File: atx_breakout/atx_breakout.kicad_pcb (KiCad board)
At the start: 2 copper layers, 90 x 60 mm, 18 parts, among them J1 Conn_02x04_Top_Bottom, J10 Screw_Terminal_01x08, J2 Conn_02x04_Top_Bottom, J3 Conn_02x04_Top_Bottom, J4 Conn_02x04_Top_Bottom, J5 ATX-24, J6 Screw_Terminal_01x08, J7 Screw_Terminal_01x08, J8 Screw_Terminal_01x08, J9 Screw_Terminal_01x08, U1 SW_DPDT_PS-70N

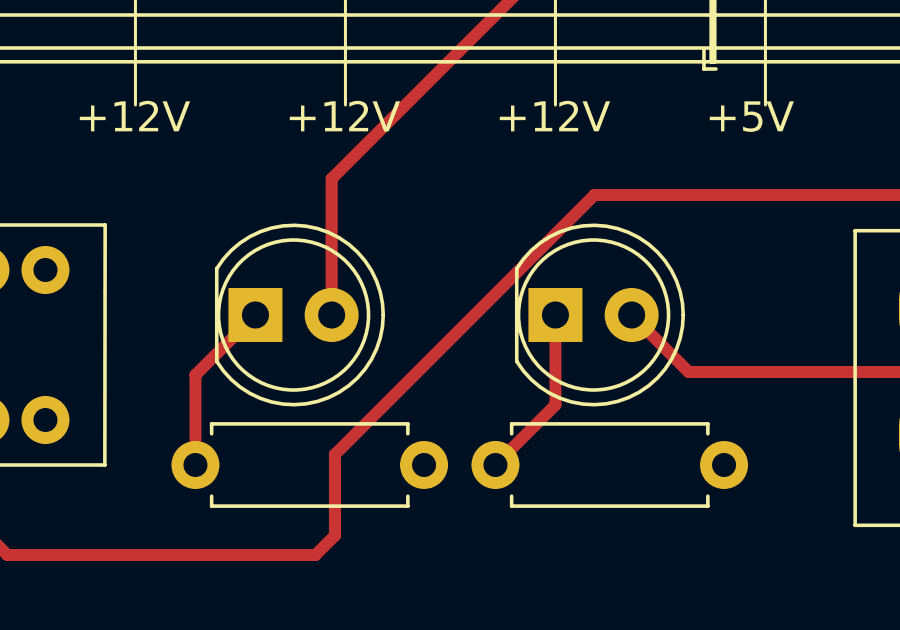
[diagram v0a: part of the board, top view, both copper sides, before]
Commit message: Update ledplane
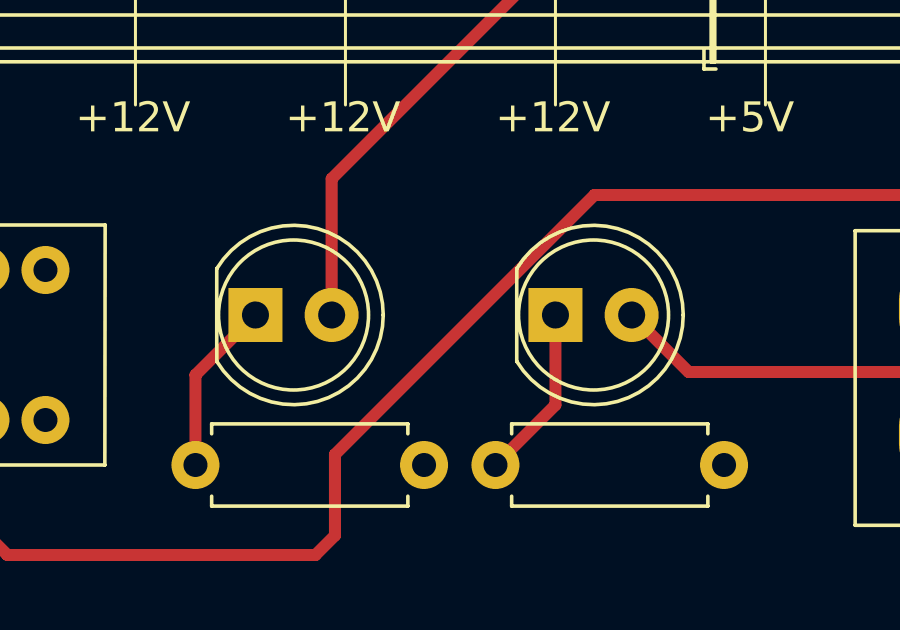
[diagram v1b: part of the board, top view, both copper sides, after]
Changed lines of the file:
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@@
 		(layer "F.Cu")
 		(at 26 17)
-		(descr "LED, diameter 5.0mm, 2 pins, http://cdn-reichelt.de/documents/datenblatt/A500/LL-504BC2E-009.pdf")
-		(tags "LED diameter 5.0mm 2 pins")
+		(descr "LED, diameter 5.0mm, 2 pins, http://cdn-reichelt.de/documents/datenblatt/A500/LL-504BC2E-009.pdf, generated by kicad-footprint-generator")
+		(tags "LED")
 		(property "Reference" "D1"
 			(at 1.27 -3.96 0)
@@
 		(fp_arc
 			(start -1.29 -1.54483)
-			(mid 2.072002 -2.880433)
-			(end 4.26 0.000462)
+			(mid 2.071756 -2.880501)
+			(end 4.26 -0.000048)
 			(stroke
 				(width 0.12)
@@
 		)
 		(fp_arc
-			(start 4.26 -0.000462)
-			(mid 2.072002 2.880433)
+			(start 4.26 0.000048)
+			(mid 2.071756 2.880501)
 			(end -1.29 1.54483)
 			(stroke
@@
 		)
 		(fp_line
-			(start -1.95 -3.25)
-			(end -1.95 3.25)
+			(start -1.94 -3.21)
+			(end -1.94 3.21)
 			(stroke
 				(width 0.05)
@@
 		)
 		(fp_line
-			(start -1.95 3.25)
-			(end 4.5 3.25)
+			(start -1.94 3.21)
+			(end 4.49 3.21)
 			(stroke
 				(width 0.05)
@@
 		)
 		(fp_line
-			(start 4.5 -3.25)
-			(end -1.95 -3.25)
+			(start 4.49 -3.21)
+			(end -1.94 -3.21)
 			(stroke
 				(width 0.05)
@@
 		)
 		(fp_line
-			(start 4.5 3.25)
-			(end 4.5 -3.25)
+			(start 4.49 3.21)
+			(end 4.49 -3.21)
 			(stroke
 				(width 0.05)
@@
 		(fp_arc
 			(start -1.23 -1.469694)
-			(mid 4.17 0.000016)
-			(end -1.230016 1.469666)
+			(mid 4.17 -0.000045)
+			(end -1.229954 1.469772)
 			(stroke
 				(width 0.1)
@@
 		(layer "F.Cu")
 		(at 16 17)
-		(descr "LED, diameter 5.0mm, 2 pins, http://cdn-reichelt.de/documents/datenblatt/A500/LL-504BC2E-009.pdf")
-		(tags "LED diameter 5.0mm 2 pins")
+		(descr "LED, diameter 5.0mm, 2 pins, http://cdn-reichelt.de/documents/datenblatt/A500/LL-504BC2E-009.pdf, generated by kicad-footprint-generator")
+		(tags "LED")
 		(property "Reference" "D2"
 			(at 1.27 -3.96 0)
@@
 		(fp_arc
 			(start -1.29 -1.54483)
-			(mid 2.072002 -2.880433)
-			(end 4.26 0.000462)
+			(mid 2.071756 -2.880501)
+			(end 4.26 -0.000048)
 			(stroke
 				(width 0.12)
@@
 		)
 		(fp_arc
-			(start 4.26 -0.000462)
-			(mid 2.072002 2.880433)
+			(start 4.26 0.000048)
+			(mid 2.071756 2.880501)
 			(end -1.29 1.54483)
 			(stroke
@@
 		)
 		(fp_line
-			(start -1.95 -3.25)
-			(end -1.95 3.25)
+			(start -1.94 -3.21)
+			(end -1.94 3.21)
 			(stroke
 				(width 0.05)
@@
 		)
 		(fp_line
-			(start -1.95 3.25)
-			(end 4.5 3.25)
+			(start -1.94 3.21)
+			(end 4.49 3.21)
 			(stroke
 				(width 0.05)
@@
 		)
 		(fp_line
-			(start 4.5 -3.25)
-			(end -1.95 -3.25)
+			(start 4.49 -3.21)
+			(end -1.94 -3.21)
 			(stroke
 				(width 0.05)
@@
 		)
 		(fp_line
-			(start 4.5 3.25)
-			(end 4.5 -3.25)
+			(start 4.49 3.21)
+			(end 4.49 -3.21)
 			(stroke
 				(width 0.05)
@@
 		(fp_arc
 			(start -1.23 -1.469694)
-			(mid 4.17 0.000016)
-			(end -1.230016 1.469666)
+			(mid 4.17 -0.000045)
+			(end -1.229954 1.469772)
 			(stroke
 				(width 0.1)
